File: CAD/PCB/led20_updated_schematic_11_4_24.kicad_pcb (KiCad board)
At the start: 2 copper layers, 71 x 40 mm, 32 parts, among them U3 Battery, U6 JST

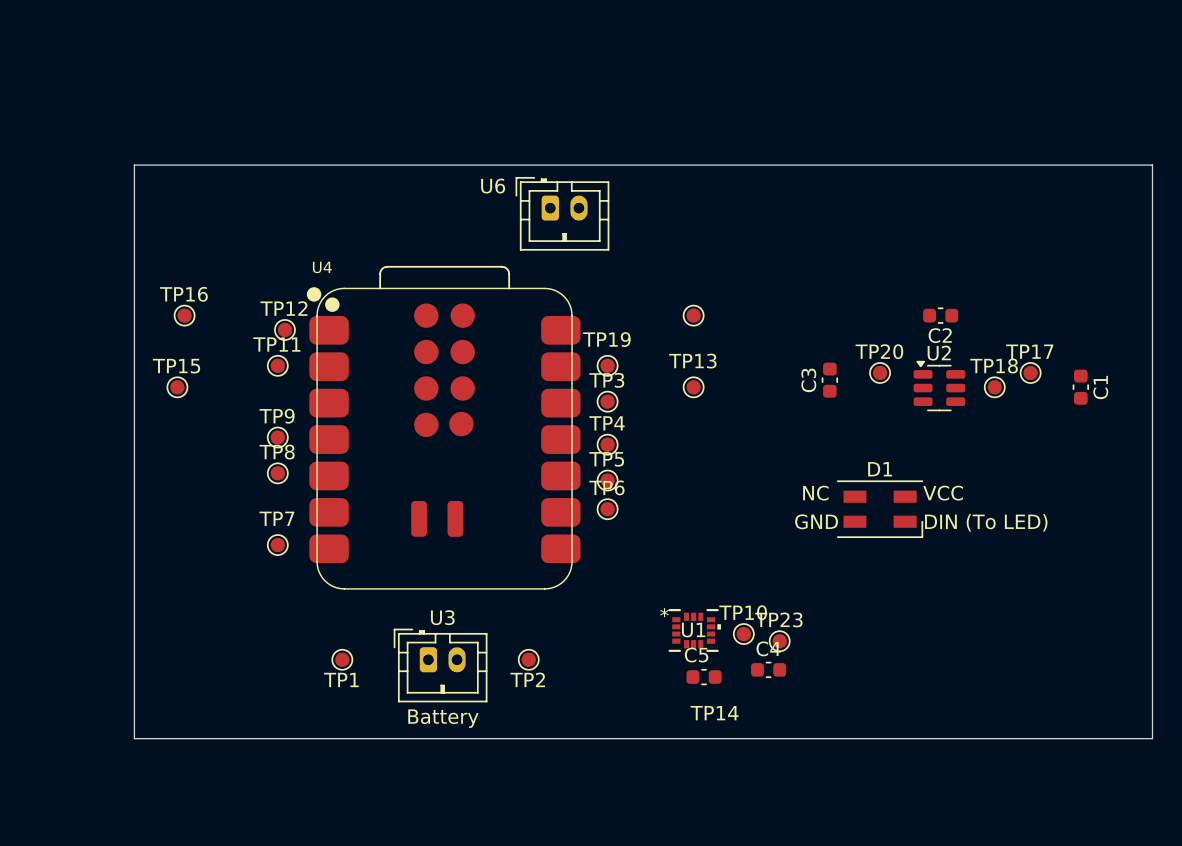
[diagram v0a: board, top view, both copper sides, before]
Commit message: Updated PCB and Schematic
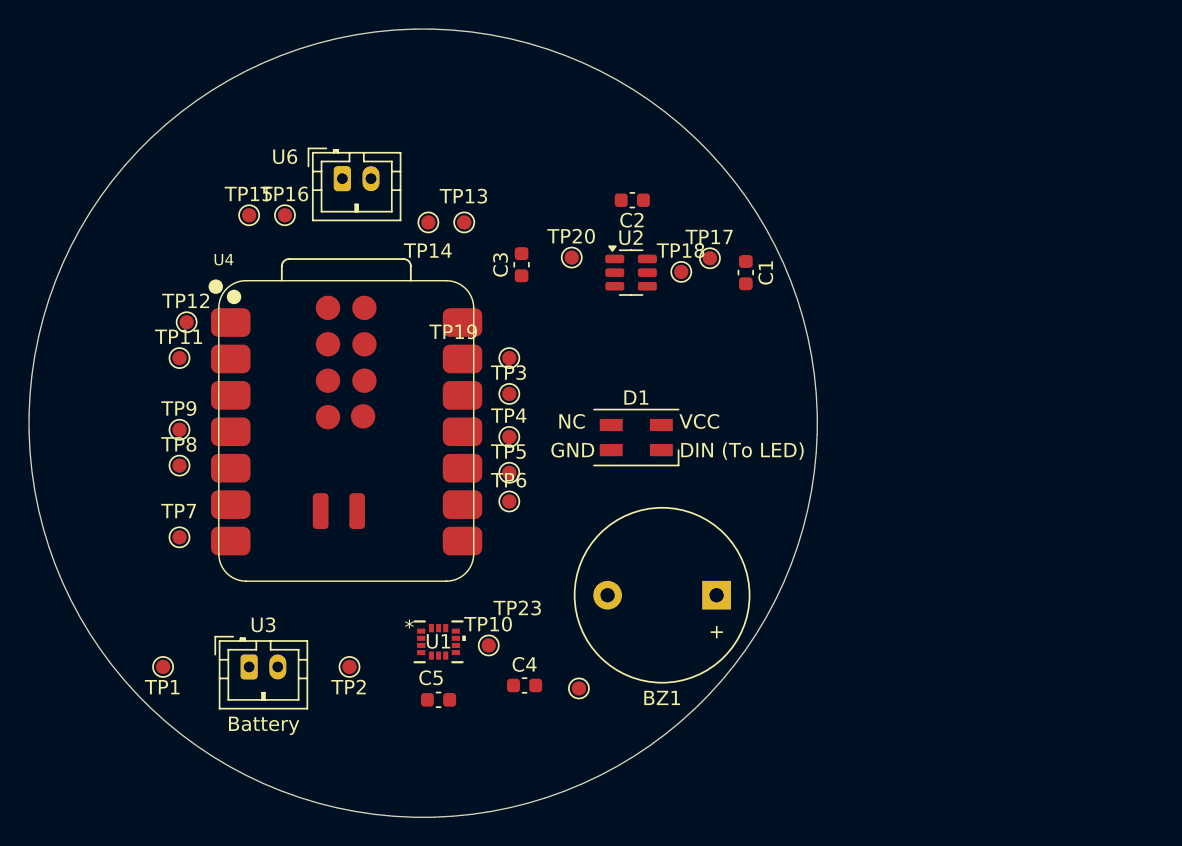
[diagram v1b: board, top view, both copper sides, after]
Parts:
- added BZ1: Piezo Buzzer, Buzzer_Beeper:Buzzer_12x9.5RM7.6, F.Cu at (163.6, 90.0)
- moved C1 24.7 mm to (165.6, 67.5)
- moved TP17 23.8 mm to (163.1, 66.5)
- moved TP18 23.3 mm to (161.1, 67.5)
- moved C2 23.0 mm to (157.7, 62.5)
- moved C3 23.0 mm to (150.0, 67.0)
- moved TP20 23.0 mm to (153.5, 66.5)
- moved U2 23.0 mm to (157.6, 67.5)
- moved TP13 19.7 mm to (146.0, 64.0)
- moved TP14 19.6 mm to (143.5, 64.0)
- moved C5 18.6 mm to (144.2, 97.3)
- moved TP10 17.8 mm to (147.7, 93.5)
- moved U1 17.8 mm to (144.2, 93.2)
- moved D1 17.7 mm to (158.0, 79.0)
- moved C4 17.0 mm to (150.2, 96.3)
- moved U6 14.6 mm to (137.5, 61.0)
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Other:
- board size 71 x 40 mm -> 55 x 55 mm
